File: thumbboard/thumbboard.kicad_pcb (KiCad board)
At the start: 2 copper layers, 79.7 x 37 mm, 6 parts, among them J1 Conn_01x05_MountingPin, SW1 SW_Push, SW2 SW_Push, SW3 SW_Push, SW4 SW_Push

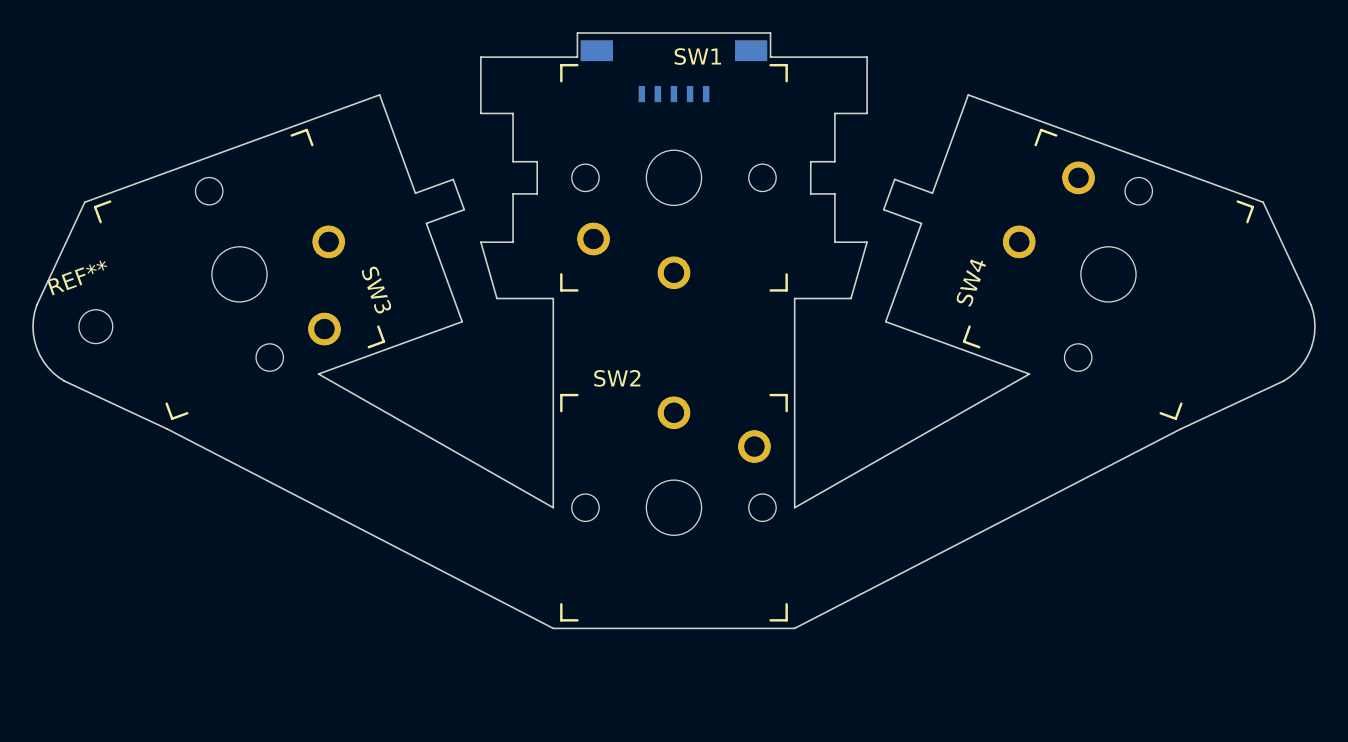
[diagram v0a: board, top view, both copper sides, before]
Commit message: sdf
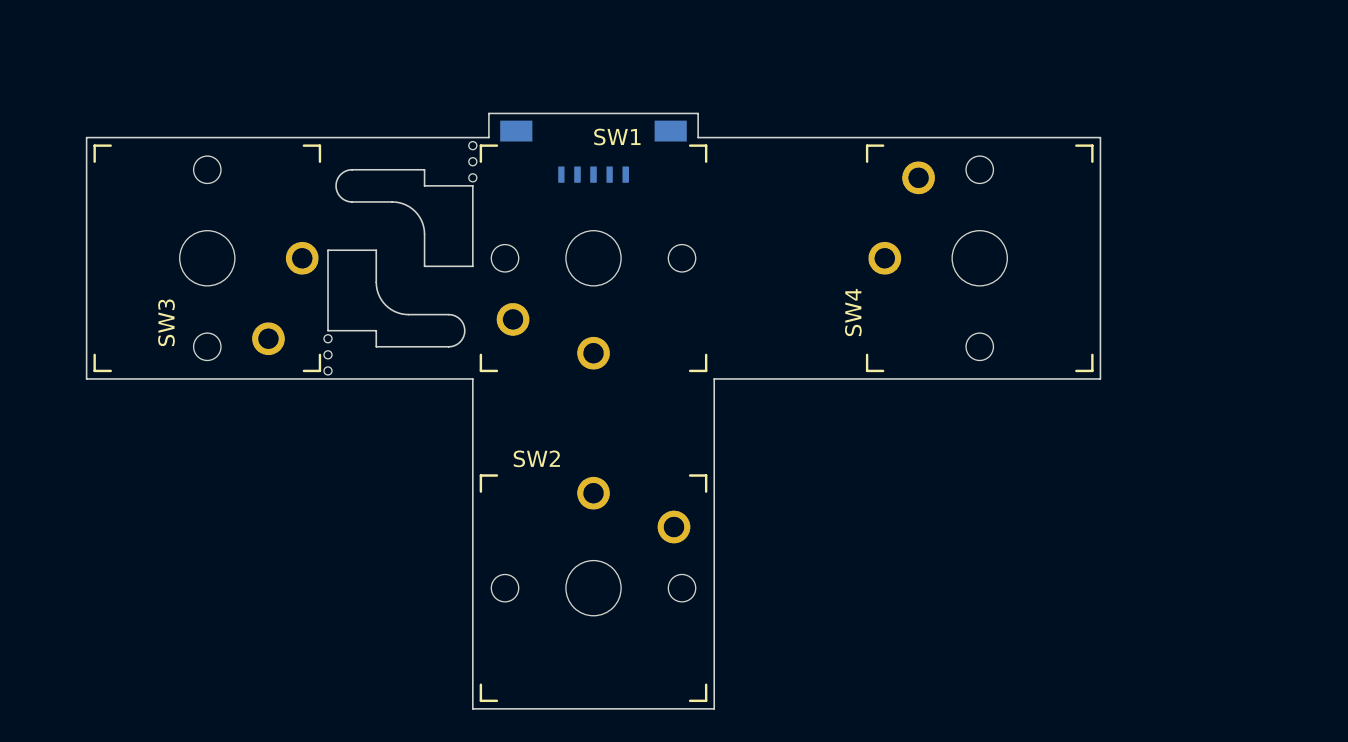
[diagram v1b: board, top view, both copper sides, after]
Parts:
- removed the REF** at (114.1, 89.2)
- added REF**: NPTH 0.5mm, panelization:NPTH 0.5mm, F.Cu at (137.5, 80.0)
- added REF**: NPTH 0.5mm, panelization:NPTH 0.5mm, F.Cu at (137.5, 79.0)
- added REF**: NPTH 0.5mm, panelization:NPTH 0.5mm, F.Cu at (137.5, 78.0)
- added REF**: NPTH 0.5mm, panelization:NPTH 0.5mm, F.Cu at (128.5, 92.0)
- added REF**: NPTH 0.5mm, panelization:NPTH 0.5mm, F.Cu at (128.5, 90.0)
- added REF**: NPTH 0.5mm, panelization:NPTH 0.5mm, F.Cu at (128.5, 91.0)
- moved SW4 8.06 mm to (169.0, 85.0), turned to -90 degrees
- moved J1 7.07 mm to (145.0, 78.9)
- moved SW1 7.07 mm to (145.0, 85.0)
- moved SW2 7.07 mm to (145.0, 105.5)
- moved SW3 2.24 mm to (121.0, 85.0), turned to 90 degrees
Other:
- board size 79.7 x 37 mm -> 63 x 37 mm
